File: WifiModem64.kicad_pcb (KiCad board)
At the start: 2 copper layers, 20 parts, among them J1 C64-UserPort, Q1 BSS138, Q2 BSS138, Q3 BSS138, Q4 BSS138, U1 WeMos_mini, U2 WeMos_D1_mini_OLED_Shield

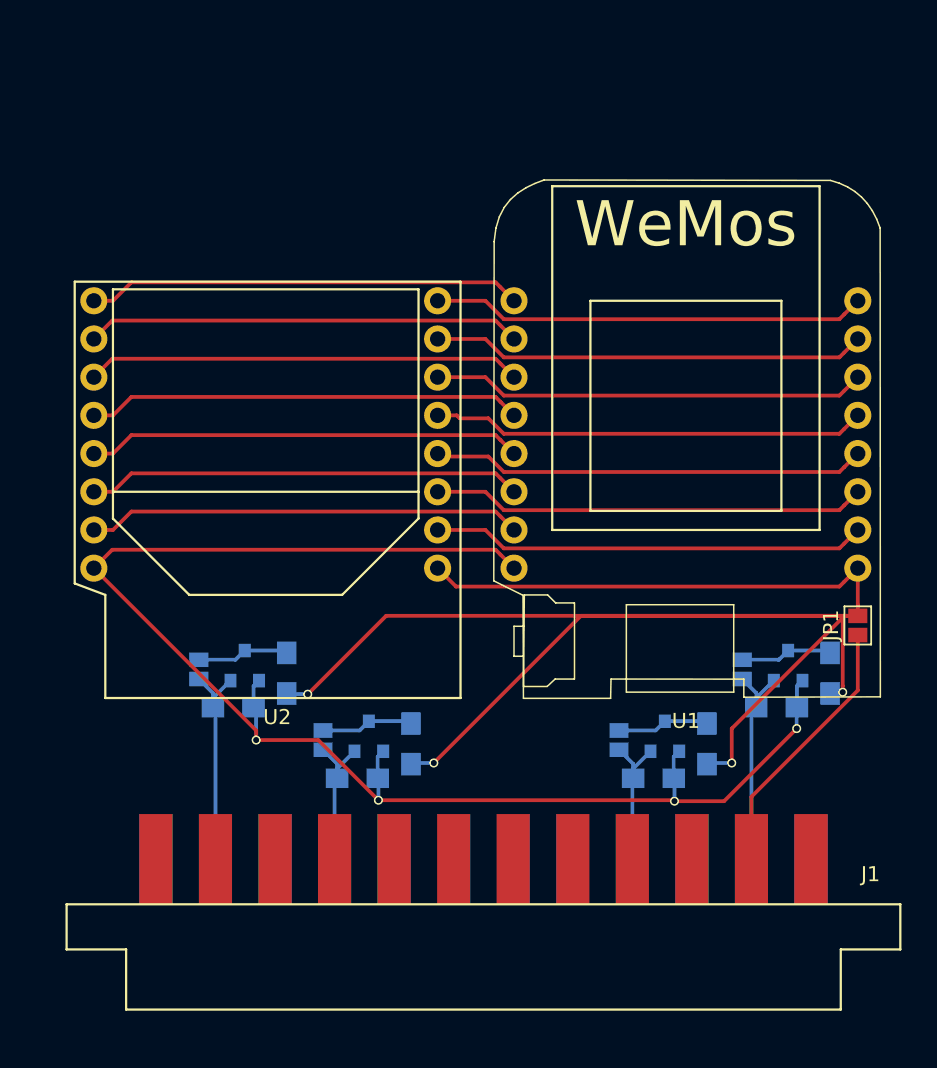
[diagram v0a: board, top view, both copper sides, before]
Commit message: WiP.
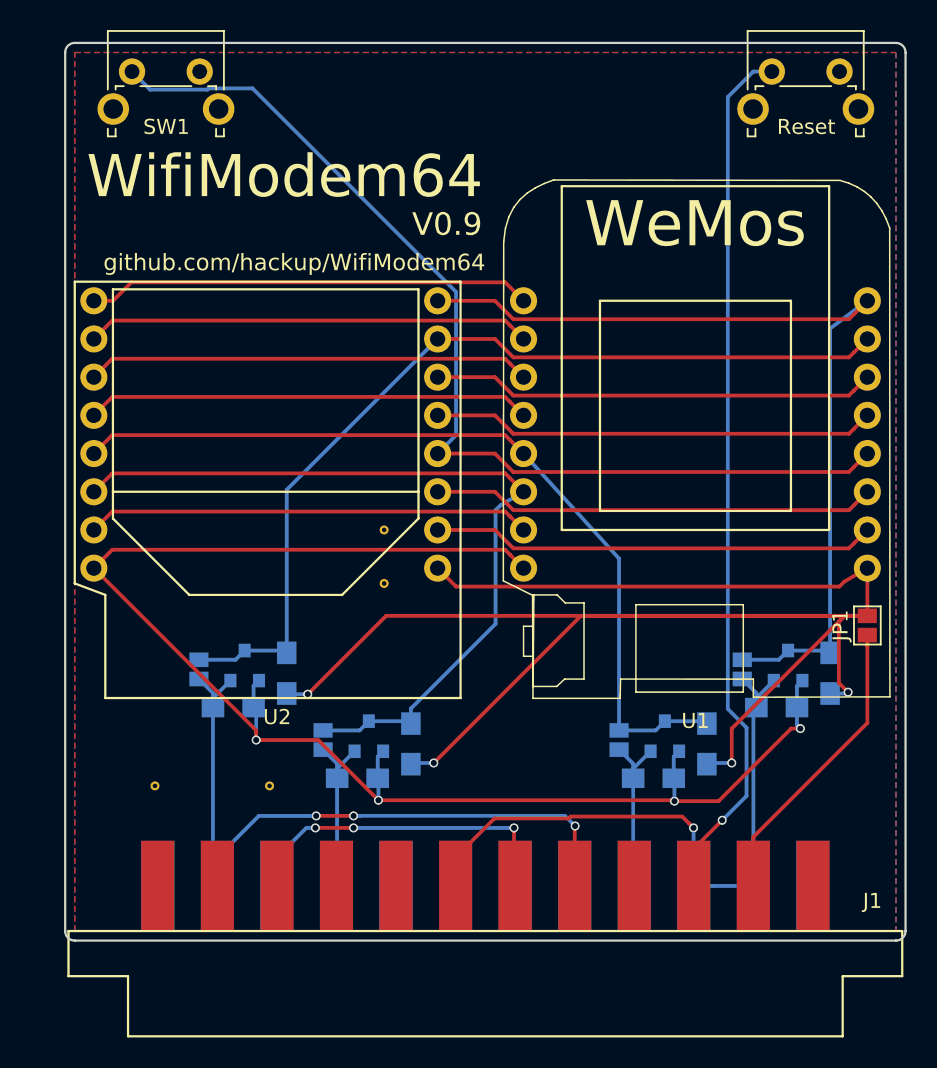
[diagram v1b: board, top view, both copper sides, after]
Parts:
- added REF**: VIA-0.6mm, hackup:VIA-0.6mm, F.Cu at (124.7, 117.3)
- added REF**: VIA-0.6mm, hackup:VIA-0.6mm, F.Cu at (132.3, 117.3)
- added REF**: VIA-0.6mm, hackup:VIA-0.6mm, F.Cu at (140.0, 103.9)
- added REF**: VIA-0.6mm, hackup:VIA-0.6mm, F.Cu at (140.0, 100.3)
- added Reset: Reset, Buttons_Switches_THT:SW_Tactile_SPST_Angled_PTS645Vx58-2LFS, F.Cu at (165.7, 69.8)
- added SW1: Push, Buttons_Switches_THT:SW_Tactile_SPST_Angled_PTS645Vx58-2LFS, F.Cu at (123.2, 69.8)
- moved J1 1.78 mm to (146.7, 127.0)
- moved JP1 0.64 mm to (172.1, 106.7)
- moved U1 0.63 mm to (160.7, 95.2)
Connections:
- J1 pad 3: Net-(J1-Pad3) -> RST
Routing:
- net RST: track 0.00 -> 58.1 mm, vias 0 -> 1
- net W_D3: track 29.0 -> 68.5 mm
- net SP1: track 14.7 -> 47.9 mm, vias 0 -> 3
- net SP2: track 14.8 -> 43.9 mm, vias 0 -> 1
- net W_RX: track 35.1 -> 60.8 mm
- net W_TX: track 35.1 -> 60.4 mm
- net Net-(J1-Pad6): track 0.00 -> 22.4 mm, vias 0 -> 3
- net W_D6: track 35.1 -> 56.6 mm
- net W_D7: track 35.1 -> 54.5 mm
- net +5V: track 127.5 -> 130.7 mm
- net Net-(J1-Pad2): track 17.8 -> 19.8 mm
- net RTS: track 10.0 -> 12.0 mm
- net CTS: track 9.97 -> 11.8 mm
- net +3V3: track 98.9 -> 99.9 mm
- net W_D2: track 29.0 -> 29.6 mm
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- added copper zone on B.Cu, net GND
- added copper zone on F.Cu, net GND
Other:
- board outline added: 55.9 x 59.7 mm
- board text added: "V0.9"
- board text added: "WifiModem64"
- board text added: "github.com/hackup/WifiModem64"
